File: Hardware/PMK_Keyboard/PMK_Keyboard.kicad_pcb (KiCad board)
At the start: 2 copper layers, 174 x 153 mm, 52 parts, among them IC1 SN74HC165PWR, IC2 SN74HC165PWR, IC3 SN74HC165PWR, IC4 SN74HC165PWR, IC5 SN74HC165PWR, IC7 ESP32-S2FH4, SW1 SW_Push, SW10 SW_Push, SW11 SW_Push, SW12 SW_Push, SW13 SW_Push, SW14 SW_Push, SW15 SW_Push, SW16 SW_Push, SW17 SW_Push, SW18 SW_Push, SW19 SW_Push, SW2 SW_Push, SW20 SW_Push, SW21 SW_Push, SW22 SW_Push, SW23 SW_Push, SW24 SW_Push, SW25 SW_Push, SW26 SW_Push, SW27 SW_Push, SW28 SW_Push, SW29 SW_Push, SW3 SW_Push, SW30 SW_Push, SW31 SW_Push, SW32 SW_Push, SW33 SW_Push, SW34 SW_Push, SW35 SW_Push, SW36 SW_Push, SW37 SW_Push, SW38 SW_Push, SW39 SW_Push, SW4 SW_Push, SW40 SW_Push, SW5 SW_Push, SW6 SW_Push, SW7 SW_Push, SW8 SW_Push, SW9 SW_Push

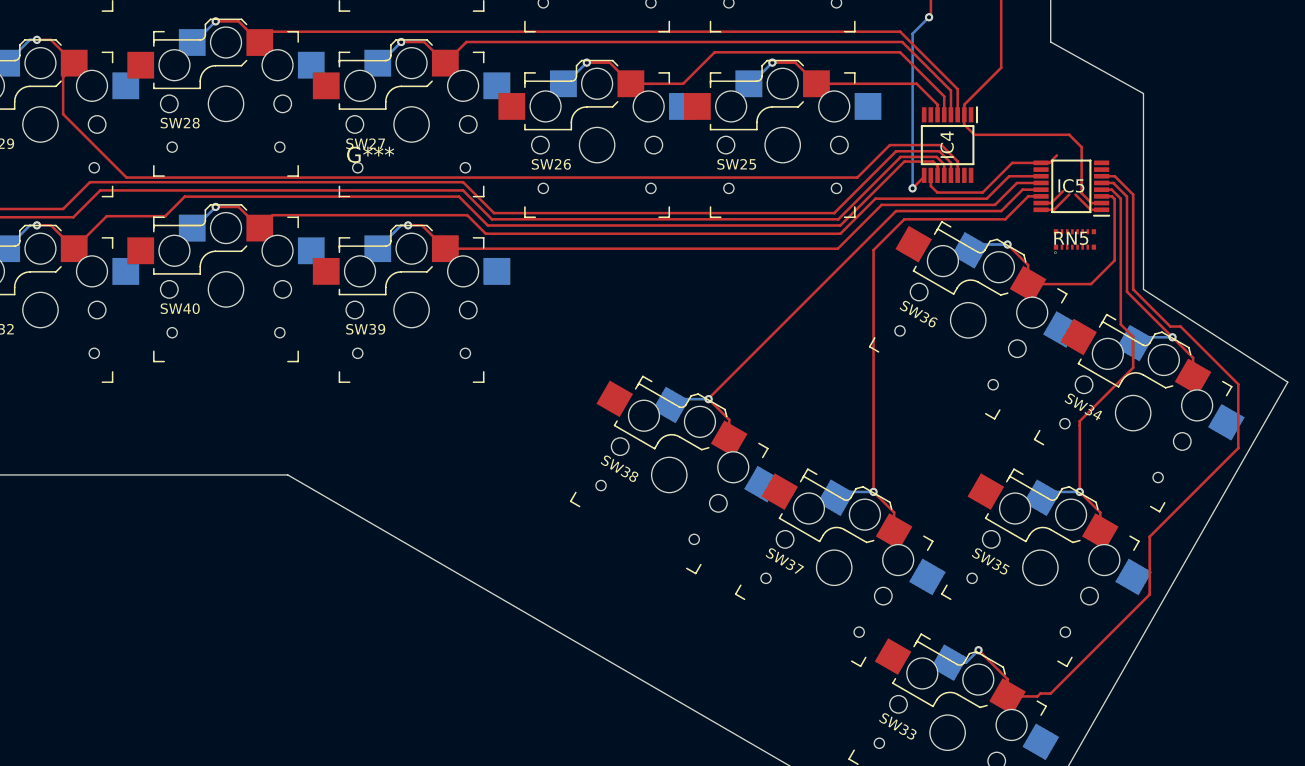
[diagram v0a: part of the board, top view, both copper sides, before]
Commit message: quick routing update
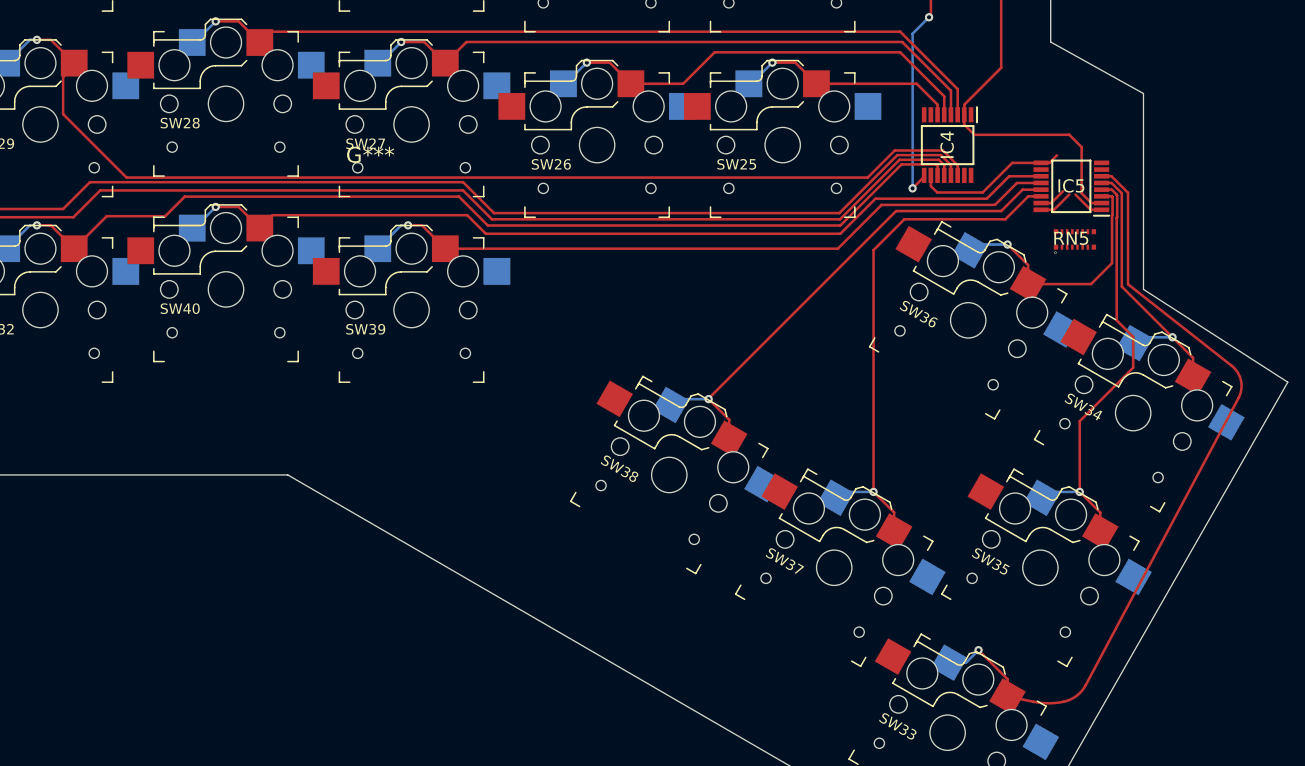
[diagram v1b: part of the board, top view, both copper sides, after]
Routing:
- net /33: track 77.9 -> 77.1 mm
- net /29: track 106.5 -> 105.8 mm
